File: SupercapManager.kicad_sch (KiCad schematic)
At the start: 9 parts, among them J1 JST4_F, J2 XT30_F, J3 XT30_F, J4 XT30_F, J5 XT30_F, Q1 BSC059N04LS6, Q2 BSC059N04LS6

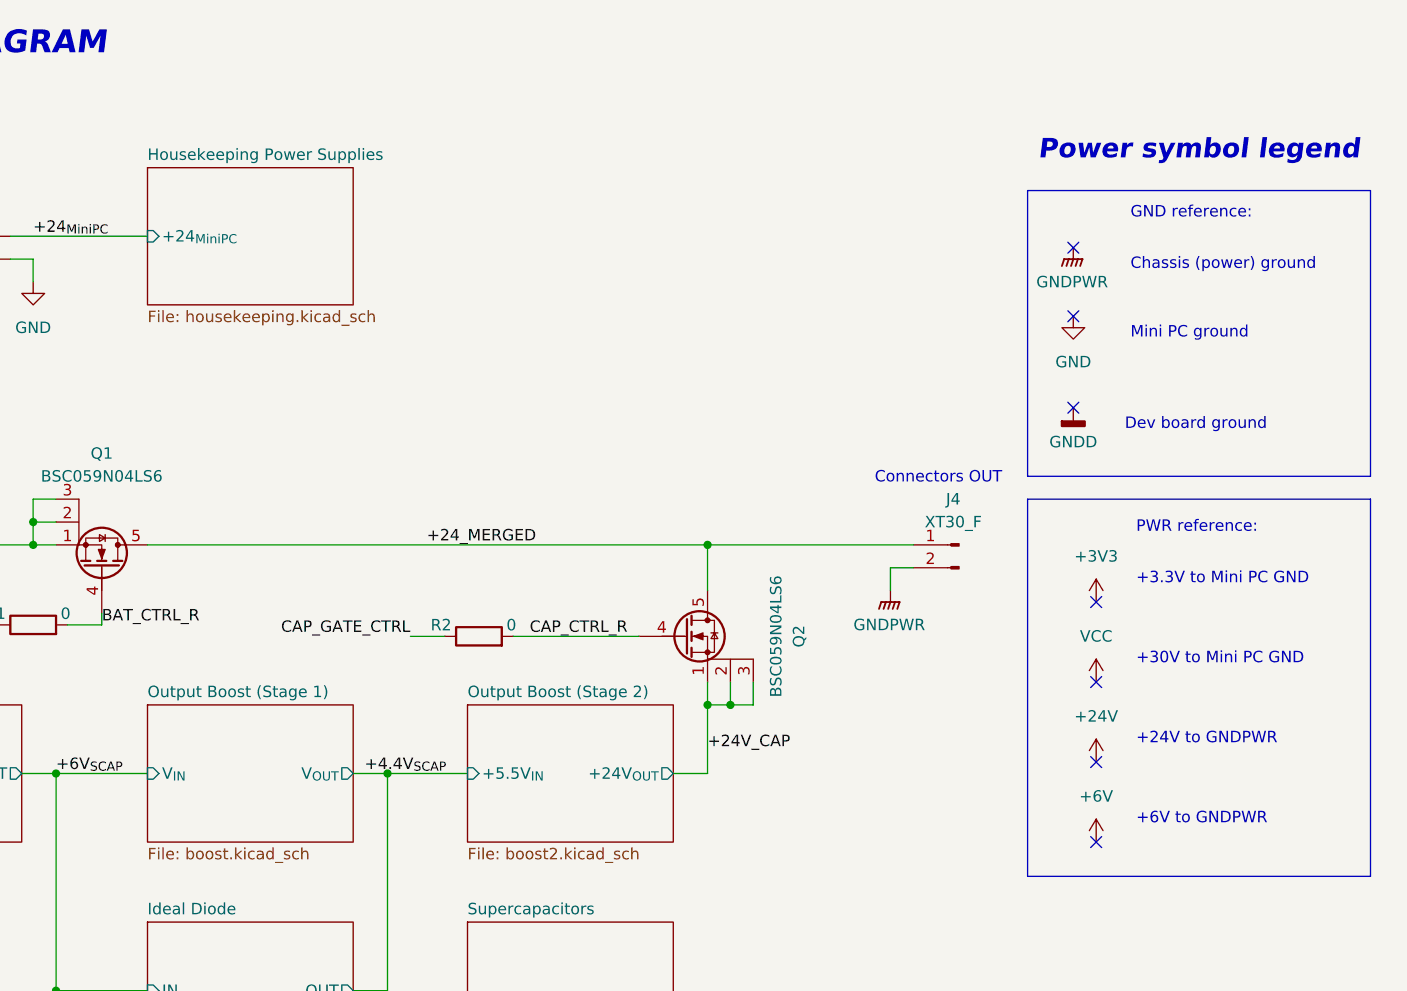
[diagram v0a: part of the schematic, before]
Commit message: Finalized design !!!
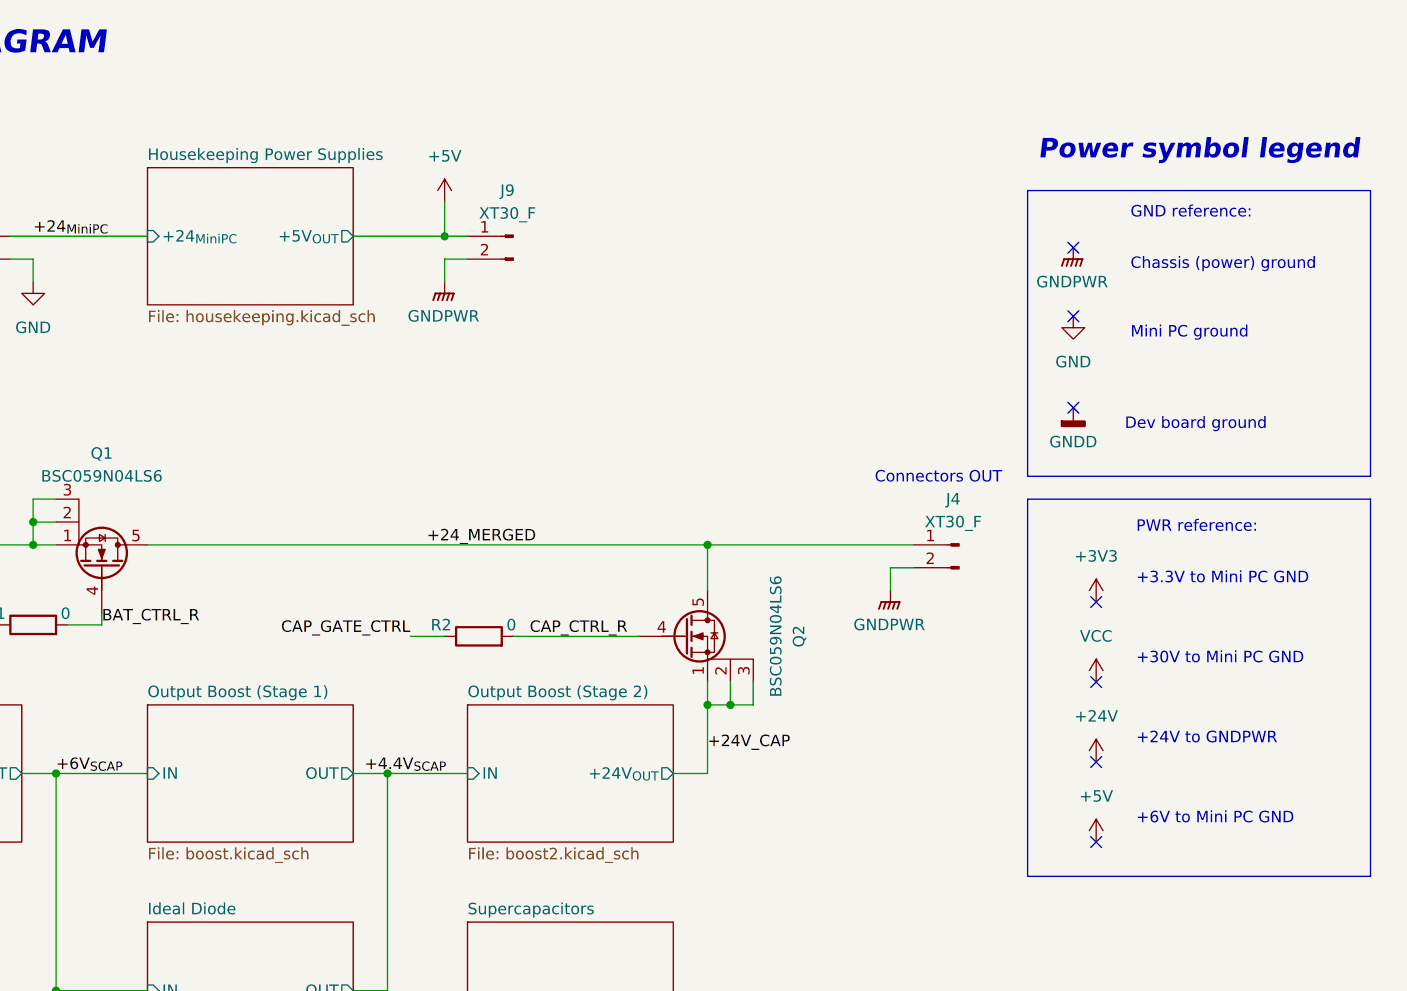
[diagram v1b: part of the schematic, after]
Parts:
- added J9: XT30_F, Connector_AMASS:AMASS_XT30U-F_1x02_P5.0mm_Vertical, symbol Connector:Conn_01x02_Pin
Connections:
- net GNDPWR: now also J9.2 (Pin_2)
- new net +5V: J9.1 (Pin_1)
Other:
- sheet Housekeeping Power Supplies ports: added +5V_{OUT}; removed none
- sheet Output Boost (Stage 1) ports: added IN, OUT; removed V_{IN}, V_{OUT}
- sheet Output Boost (Stage 2) ports: added IN; removed +5.5V_{IN}
- note added: "+6V to Mini PC GND"
- note removed: "+6V to GNDPWR"
